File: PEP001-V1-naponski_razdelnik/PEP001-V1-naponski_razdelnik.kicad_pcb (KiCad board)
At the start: 2 copper layers, 45 x 45 mm, 12 parts, among them J1 Screw_Terminal_01x02

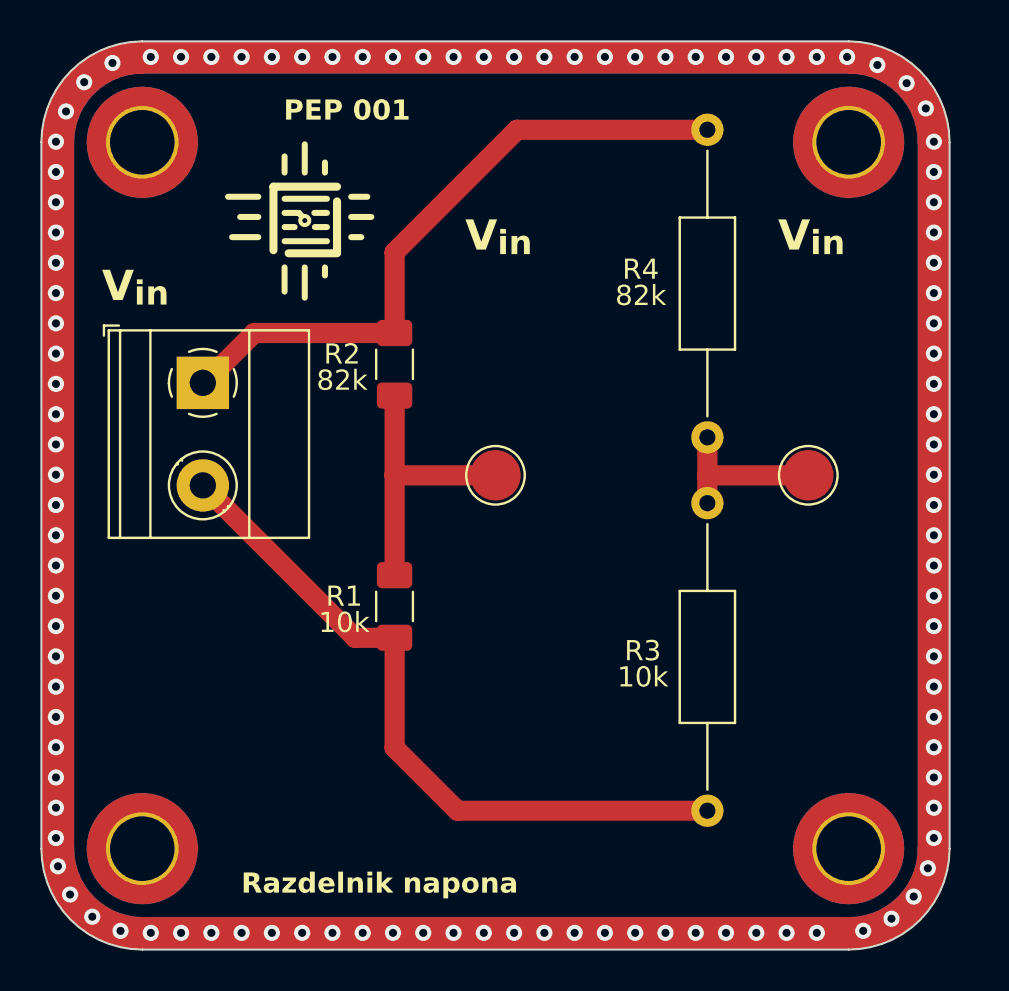
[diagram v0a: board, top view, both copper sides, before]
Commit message: Update 1,2,3,4,5,7, lib.
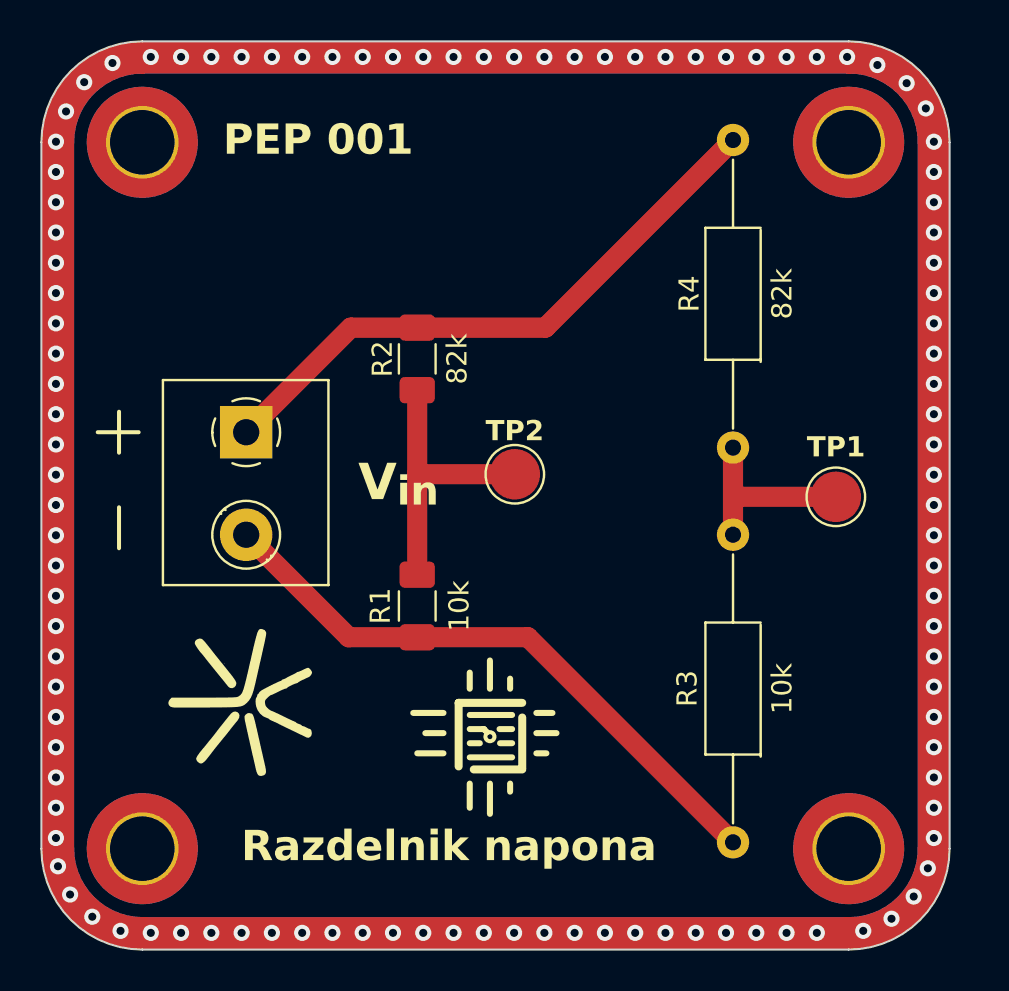
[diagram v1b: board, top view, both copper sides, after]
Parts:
- added REF**: LOGO, PEP_library:petnica_logo, F.Cu at (113.9, 93.8)
- J1: value Screw_Terminal_01x02 -> Klema; footprint TerminalBlock_Phoenix:TerminalBlock_Phoenix_MKDS-1,5-2-5.08_1x02_P5.08mm_Horizontal -> PEP_library:TerminalBlock_Phoenix_MKDS-1,5-2-5.08_1x02_P5.08mm_Horizontal
- R1, R2: footprint Resistor_SMD:R_1206_3216Metric_Pad1.30x1.75mm_HandSolder -> PEP_library:R_smd_1206
- R3, R4: footprint Resistor_THT:R_Axial_DIN0207_L6.3mm_D2.5mm_P15.24mm_Horizontal -> PEP_library:R_Axial_DIN0207_L6.3mm_D2.5mm_P15.24mm_Horizontal
- moved REF** 27.2 mm to (126.2, 95.5)
- moved R4 14.8 mm to (138.3, 65.9), turned to -90 degrees
- moved J1 3.25 mm to (114.1, 80.4)
- moved R3 2.02 mm to (138.3, 85.4)
- moved TP1 1.73 mm to (143.4, 83.6)
- moved R2 1.16 mm to (122.6, 76.7)
- moved R1 1.12 mm to (122.6, 89.0)
- moved TP2 0.96 mm to (127.5, 82.4)
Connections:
- R4 pad 1: Net-(R3-Pad1) -> 9V
- R4 pad 2: 9V -> Net-(R3-Pad1)
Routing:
- net 0: track 34.9 -> 30.4 mm
- net 9V: track 32.5 -> 30.1 mm
- net Net-(R3-Pad1): track 8.76 -> 9.36 mm
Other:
- board text added: "TP1"
- board text added: "TP2"
- board text removed: "V_{in}"
